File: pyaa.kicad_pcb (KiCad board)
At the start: 2 copper layers, 123 x 80.1 mm, 18 parts, among them J1 MJ-4PP-9, K0 KEYSW, K1 KEYSW, SW1 SW_PUSH, U1 ProMicro

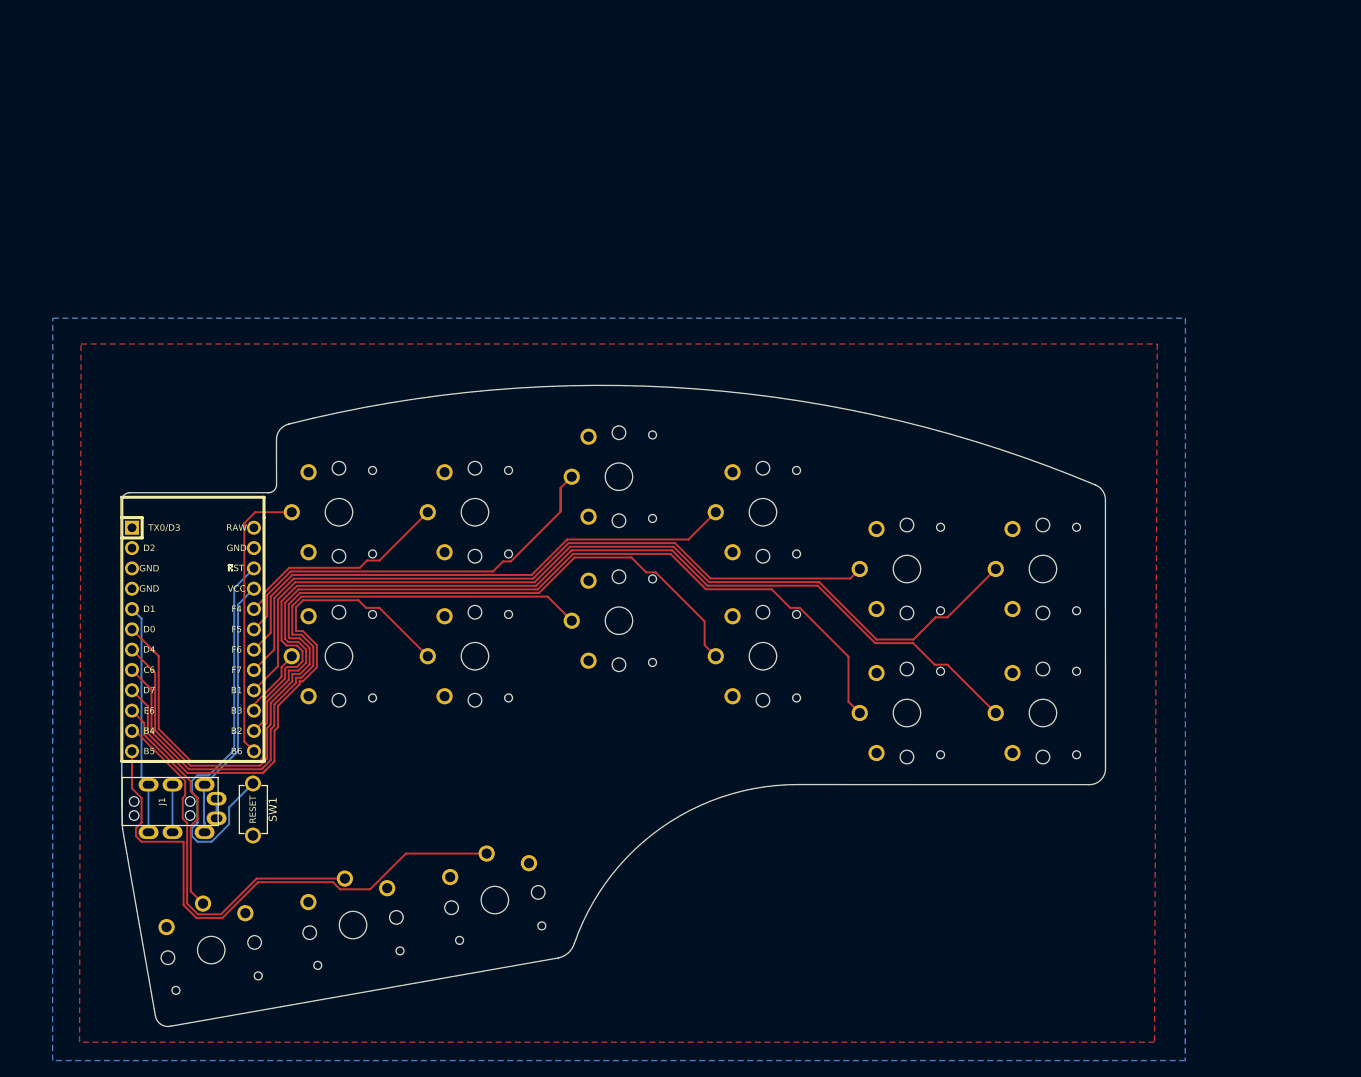
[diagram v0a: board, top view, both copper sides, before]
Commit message: Add files via upload
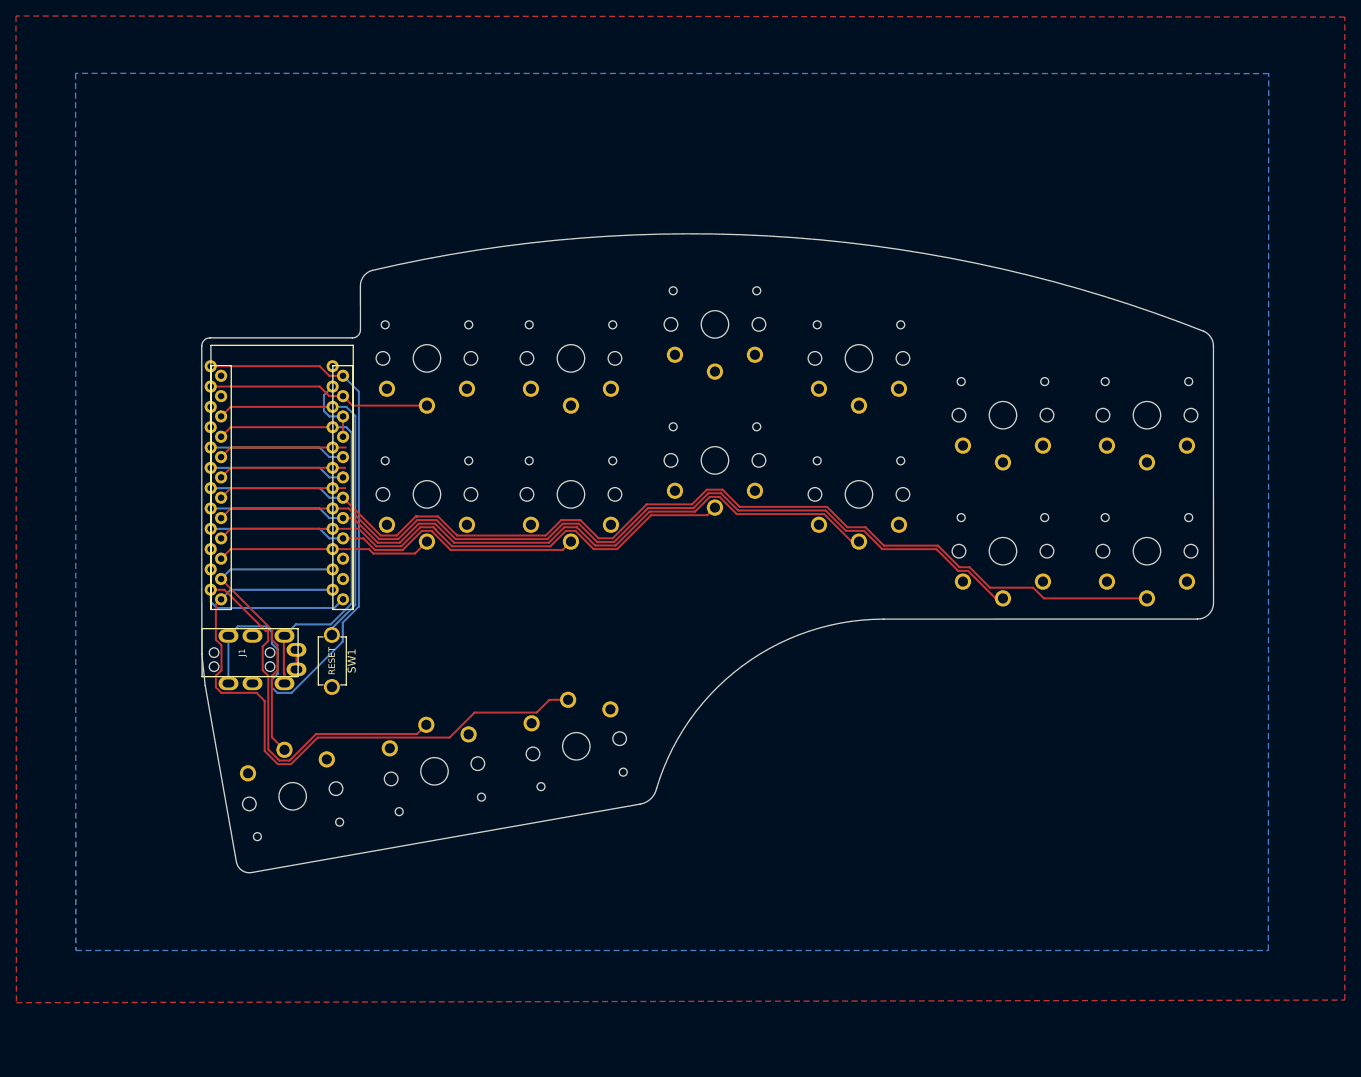
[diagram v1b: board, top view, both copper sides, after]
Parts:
- U1: footprint Keebio-Parts:ArduinoProMicro -> Lily58-footprint:ProMicro_rev2
- moved K1 24.0 mm to (209.8, 99.3), turned to 0 degrees
- moved KKL1 23.5 mm to (173.8, 92.2), turned to 0 degrees
- moved KRL1 23.5 mm to (137.8, 92.2), turned to 0 degrees
- moved KS2 23.5 mm to (191.8, 99.3), turned to 0 degrees
- moved KWL1 23.4 mm to (155.8, 88.0), turned to 0 degrees
- moved K0 23.2 mm to (209.8, 82.3), turned to 0 degrees
- moved KST2 23.0 mm to (119.8, 92.2), turned to 0 degrees
- moved KHL1 22.7 mm to (137.8, 75.2), turned to 0 degrees
- moved KTL1 22.7 mm to (173.8, 75.2), turned to 0 degrees
- moved KS1 22.7 mm to (191.8, 82.3), turned to 0 degrees
- moved KPL1 22.5 mm to (155.8, 71.0), turned to 0 degrees
- moved U1 22.3 mm to (101.5, 91.0), turned to 0 degrees
- moved KST1 22.2 mm to (119.8, 75.2), turned to 0 degrees
- moved KN1 21.7 mm to (138.4, 123.7)
- moved KA1 21.7 mm to (120.7, 126.8)
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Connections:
- U1 pad 1: Net-(U1-Pad1) -> Net-(J1-PadB)
- U1 pad 10: Net-(KO1-Pad1) -> Net-(U1-Pad10)
- U1 pad 11: Net-(KA1-Pad1) -> Net-(U1-Pad11)
- U1 pad 12: Net-(KN1-Pad1) -> Net-(KA1-Pad1)
- U1 pad 13: Net-(KST1-Pad1) -> Net-(KN1-Pad1)
- U1 pad 14: Net-(K1-Pad1) -> Net-(KO1-Pad1)
- U1 pad 16: Net-(K0-Pad1) -> Net-(KWL1-Pad1)
- U1 pad 17: Net-(KS1-Pad1) -> Net-(KS2-Pad1)
- U1 pad 18: Net-(KTL1-Pad1) -> Net-(K0-Pad1)
- U1 pad 19: Net-(KPL1-Pad1) -> Net-(KTL1-Pad1)
- U1 pad 2: Net-(U1-Pad2) -> Net-(KST1-Pad1)
- U1 pad 5: Net-(J1-PadB) -> Net-(KPL1-Pad1)
- U1 pad 6: Net-(KS2-Pad1) -> Net-(KS1-Pad1)
- U1 pad 7: Net-(KKL1-Pad1) -> Net-(K1-Pad1)
- U1 pad 8: Net-(KWL1-Pad1) -> Net-(KKL1-Pad1)
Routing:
- net Net-(K0-Pad1): track 113.5 -> 16.0 mm
- net Net-(KS1-Pad1): track 88.4 -> 17.0 mm
- net Net-(J1-PadB): track 28.8 -> 83.4 mm
- net Net-(KTL1-Pad1): track 67.5 -> 16.0 mm
- net Net-(KPL1-Pad1): track 53.9 -> 17.0 mm
- net Net-(KS2-Pad1): track 138.8 -> 111.5 mm
- net Net-(KKL1-Pad1): track 114.0 -> 91.4 mm
- net VDD: track 33.1 -> 54.6 mm
- net Net-(KRL1-Pad1): track 68.0 -> 48.6 mm
- net Net-(KST2-Pad1): track 8.76 -> 27.1 mm
- net Net-(KA1-Pad1): track 47.4 -> 65.7 mm
- net Net-(KWL1-Pad1): track 86.5 -> 69.0 mm
- net Net-(KN1-Pad1): track 68.1 -> 81.3 mm
- net Net-(KO1-Pad1): track 28.5 -> 39.7 mm
- net Net-(KHL1-Pad1): track 27.2 -> 16.1 mm
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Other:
- board size 123 x 80.1 mm -> 126.5 x 79.9 mm
